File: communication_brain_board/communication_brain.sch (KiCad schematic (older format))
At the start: 27 parts, among them J1 UART, J2 Batt, J3 RS485, J4 CAN, SW1 Reset, SW2 Programm, U1 LM2576HVT-ADJ, U2 L78L33_TO92, U3 ESP-12E, U4 MAX485E, U5 MCP2515-xSO

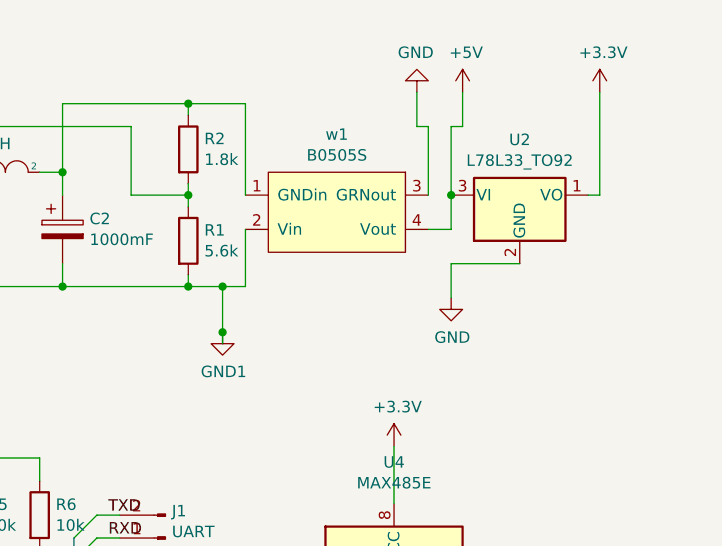
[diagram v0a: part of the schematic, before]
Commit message: fixed scheme
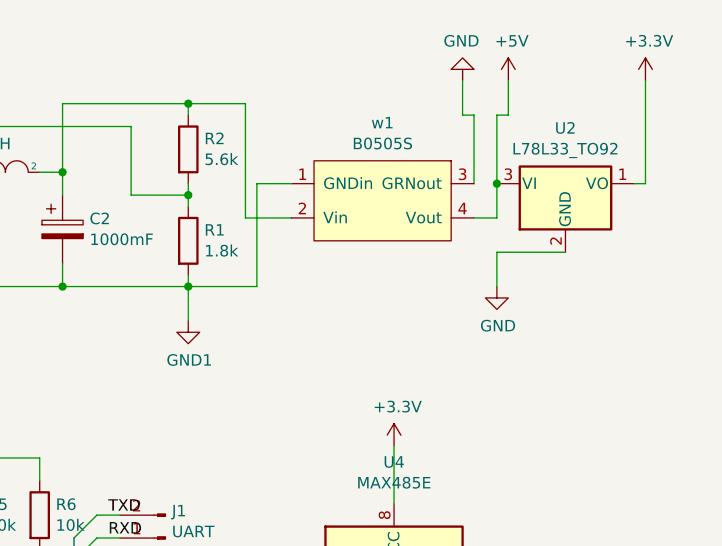
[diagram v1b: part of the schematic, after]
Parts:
- R1: value 5.6k -> 1.8k
- R2: value 1.8k -> 5.6k
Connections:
- net -BATT: now also w1.1 (GNDin); no longer w1.2 (Vin)
- net at C2.1, L1.2, R2.1: now also w1.2 (Vin); no longer w1.1 (GNDin)
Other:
- moved on the sheet: U2, w1
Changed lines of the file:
@@
 P 5500 2100
 F 0 "R1" H 5570 2146 50  0000 L CNN
-F 1 "5.6k" H 5570 2055 50  0000 L CNN
+F 1 "1.8k" H 5570 2055 50  0000 L CNN
 F 2 "Resistor_THT:R_Axial_DIN0207_L6.3mm_D2.5mm_P10.16mm_Horizontal" V 5430 2100 50  0001 C CNN
 F 3 "~" H 5500 2100 50  0001 C CNN
@@
 P 5500 1700
 F 0 "R2" H 5570 1746 50  0000 L CNN
-F 1 "1.8k" H 5570 1655 50  0000 L CNN
+F 1 "5.6k" H 5570 1655 50  0000 L CNN
 F 2 "Resistor_THT:R_Axial_DIN0207_L6.3mm_D2.5mm_P10.16mm_Horizontal" V 5430 1700 50  0001 C CNN
 F 3 "~" H 5500 1700 50  0001 C CNN
@@
 L power:GND1 #PWR0112
 U 1 1 6074119C
-P 5650 2500
-F 0 "#PWR0112" H 5650 2250 50  0001 C CNN
-F 1 "GND1" H 5655 2327 50  0000 C CNN
-F 2 "" H 5650 2500 50  0001 C CNN
-F 3 "" H 5650 2500 50  0001 C CNN
-	1    5650 2500
-	1    0    0    -1
-$EndComp
-Wire Wire Line
-	7300 1900 7300 1450
-Wire Wire Line
-	7250 1900 7300 1900
+P 5500 2450
+F 0 "#PWR0112" H 5500 2200 50  0001 C CNN
+F 1 "GND1" H 5505 2277 50  0000 C CNN
+F 2 "" H 5500 2450 50  0001 C CNN
+F 3 "" H 5500 2450 50  0001 C CNN
+	1    5500 2450
+	1    0    0    -1
+$EndComp
+Wire Wire Line
+	7500 1850 7500 1400
+Wire Wire Line
+	7450 1850 7500 1850
 $Comp
 L power:+3.3V #PWR0105
 U 1 1 600626C6
-P 7300 1450
-F 0 "#PWR0105" H 7300 1300 50  0001 C CNN
-F 1 "+3.3V" H 7315 1623 50  0000 C CNN
-F 2 "" H 7300 1450 50  0001 C CNN
-F 3 "" H 7300 1450 50  0001 C CNN
-	1    7300 1450
+P 7500 1400
+F 0 "#PWR0105" H 7500 1250 50  0001 C CNN
+F 1 "+3.3V" H 7515 1573 50  0000 C CNN
+F 2 "" H 7500 1400 50  0001 C CNN
+F 3 "" H 7500 1400 50  0001 C CNN
+	1    7500 1400
 	1    0    0    -1
 $EndComp
@@
 L Regulator_Linear:L78L33_TO92 U2
 U 1 1 6005D69D
-P 6950 1900
-F 0 "U2" H 6950 2142 50  0000 C CNN
-F 1 "L78L33_TO92" H 6950 2051 50  0000 C CNN
-F 2 "Package_TO_SOT_THT:TO-92_Inline" H 6950 2125 50  0001 C CIN
-F 3 "http://www.st.com/content/ccc/resource/technical/document/datasheet/15/55/e5/aa/23/5b/43/fd/CD00000446.pdf/files/CD00000446.pdf/jcr:content/translations/en.CD00000446.pdf" H 6950 1850 50  0001 C CNN
-	1    6950 1900
+P 7150 1850
+F 0 "U2" H 7150 2092 50  0000 C CNN
+F 1 "L78L33_TO92" H 7150 2001 50  0000 C CNN
+F 2 "Package_TO_SOT_THT:TO-92_Inline" H 7150 2075 50  0001 C CIN
+F 3 "http://www.st.com/content/ccc/resource/technical/document/datasheet/15/55/e5/aa/23/5b/43/fd/CD00000446.pdf/files/CD00000446.pdf/jcr:content/translations/en.CD00000446.pdf" H 7150 1800 50  0001 C CNN
+	1    7150 1850
 	1    0    0    -1
 $EndComp
@@
 L power:+5V #PWR0104
 U 1 1 6005BBEE
-P 6700 1450
-F 0 "#PWR0104" H 6700 1300 50  0001 C CNN
-F 1 "+5V" H 6715 1623 50  0000 C CNN
-F 2 "" H 6700 1450 50  0001 C CNN
-F 3 "" H 6700 1450 50  0001 C CNN
-	1    6700 1450
+P 6900 1400
+F 0 "#PWR0104" H 6900 1250 50  0001 C CNN
+F 1 "+5V" H 6915 1573 50  0000 C CNN
+F 2 "" H 6900 1400 50  0001 C CNN
+F 3 "" H 6900 1400 50  0001 C CNN
+	1    6900 1400
 	1    0    0    -1
 $EndComp
@@
 L power:GND #PWR0103
 U 1 1 60032A9B
-P 6650 2350
-F 0 "#PWR0103" H 6650 2100 50  0001 C CNN
-F 1 "GND" H 6655 2177 50  0000 C CNN
-F 2 "" H 6650 2350 50  0001 C CNN
-F 3 "" H 6650 2350 50  0001 C CNN
-	1    6650 2350
+P 6850 2300
+F 0 "#PWR0103" H 6850 2050 50  0001 C CNN
+F 1 "GND" H 6855 2127 50  0000 C CNN
+F 2 "" H 6850 2300 50  0001 C CNN
+F 3 "" H 6850 2300 50  0001 C CNN
+	1    6850 2300
 	1    0    0    -1
 $EndComp
@@
 L Converter_DCDC:B0505S w1
 U 1 1 606C6681
-P 6150 1750
-F 0 "w1" H 6150 1865 50  0000 C CNN
-F 1 "B0505S" H 6150 1774 50  0000 C CNN
-F 2 "" H 6150 1750 50  0001 C CNN
-F 3 "" H 6150 1750 50  0001 C CNN
-	1    6150 1750
-	1    0    0    -1
-$EndComp
-Wire Wire Line
-	6550 2050 6650 2050
-Wire Wire Line
-	6650 2050 6650 1900
-Wire Wire Line
-	6950 2200 6650 2200
-Wire Wire Line
-	6650 2200 6650 2350
+P 6350 1700
+F 0 "w1" H 6350 1815 50  0000 C CNN
+F 1 "B0505S" H 6350 1724 50  0000 C CNN
+F 2 "" H 6350 1700 50  0001 C CNN
+F 3 "" H 6350 1700 50  0001 C CNN
+	1    6350 1700
+	1    0    0    -1
+$EndComp
+Wire Wire Line
+	6750 2000 6850 2000
+Wire Wire Line
+	6850 2000 6850 1850
+Wire Wire Line
+	7150 2150 6850 2150
+Wire Wire Line
+	6850 2150 6850 2300
 $Comp
 L power:GND #PWR0113
 U 1 1 607A766E
-P 6500 1450
-F 0 "#PWR0113" H 6500 1200 50  0001 C CNN
-F 1 "GND" H 6505 1277 50  0000 C CNN
-F 2 "" H 6500 1450 50  0001 C CNN
-F 3 "" H 6500 1450 50  0001 C CNN
-	1    6500 1450
+P 6700 1400
+F 0 "#PWR0113" H 6700 1150 50  0001 C CNN
+F 1 "GND" H 6705 1227 50  0000 C CNN
+F 2 "" H 6700 1400 50  0001 C CNN
+F 3 "" H 6700 1400 50  0001 C CNN
+	1    6700 1400
 	-1   0    0    1
 $EndComp
 Wire Wire Line
-	6550 1900 6550 1600
-Wire Wire Line
-	6550 1600 6500 1600
-Wire Wire Line
-	6500 1600 6500 1450
-Wire Wire Line
-	6650 1900 6650 1600
-Wire Wire Line
-	6650 1600 6700 1600
-Wire Wire Line
-	6700 1600 6700 1450
-Connection ~ 6650 1900
-Wire Wire Line
-	5750 2050 5750 2300
-Wire Wire Line
-	5650 2300 5500 2300
+	6750 1850 6750 1550
+Wire Wire Line
+	6750 1550 6700 1550
+Wire Wire Line
+	6700 1550 6700 1400
+Wire Wire Line
+	6850 1850 6850 1550
+Wire Wire Line
+	6850 1550 6900 1550
+Wire Wire Line
+	6900 1550 6900 1400
+Connection ~ 6850 1850
 Connection ~ 5500 2300
-Wire Wire Line
-	5650 2550 5650 2500
-Connection ~ 5650 2500
-Wire Wire Line
-	5650 2500 5650 2300
-Wire Wire Line
-	5750 1900 5750 1500
 Connection ~ 5500 1500
 Wire Wire Line
-	5750 2300 5650 2300
-Connection ~ 5650 2300
-Wire Wire Line
 	5500 1500 5750 1500
+Wire Wire Line
+	5950 2000 5750 2000
+Wire Wire Line
+	5750 2000 5750 1500
+Wire Wire Line
+	5950 1850 5800 1850
+Wire Wire Line
+	5800 1850 5800 2300
+Wire Wire Line
+	5500 2300 5800 2300
+Wire Wire Line
+	5500 2450 5500 2300
 Wire Bus Line
 	4700 3550 4700 4200

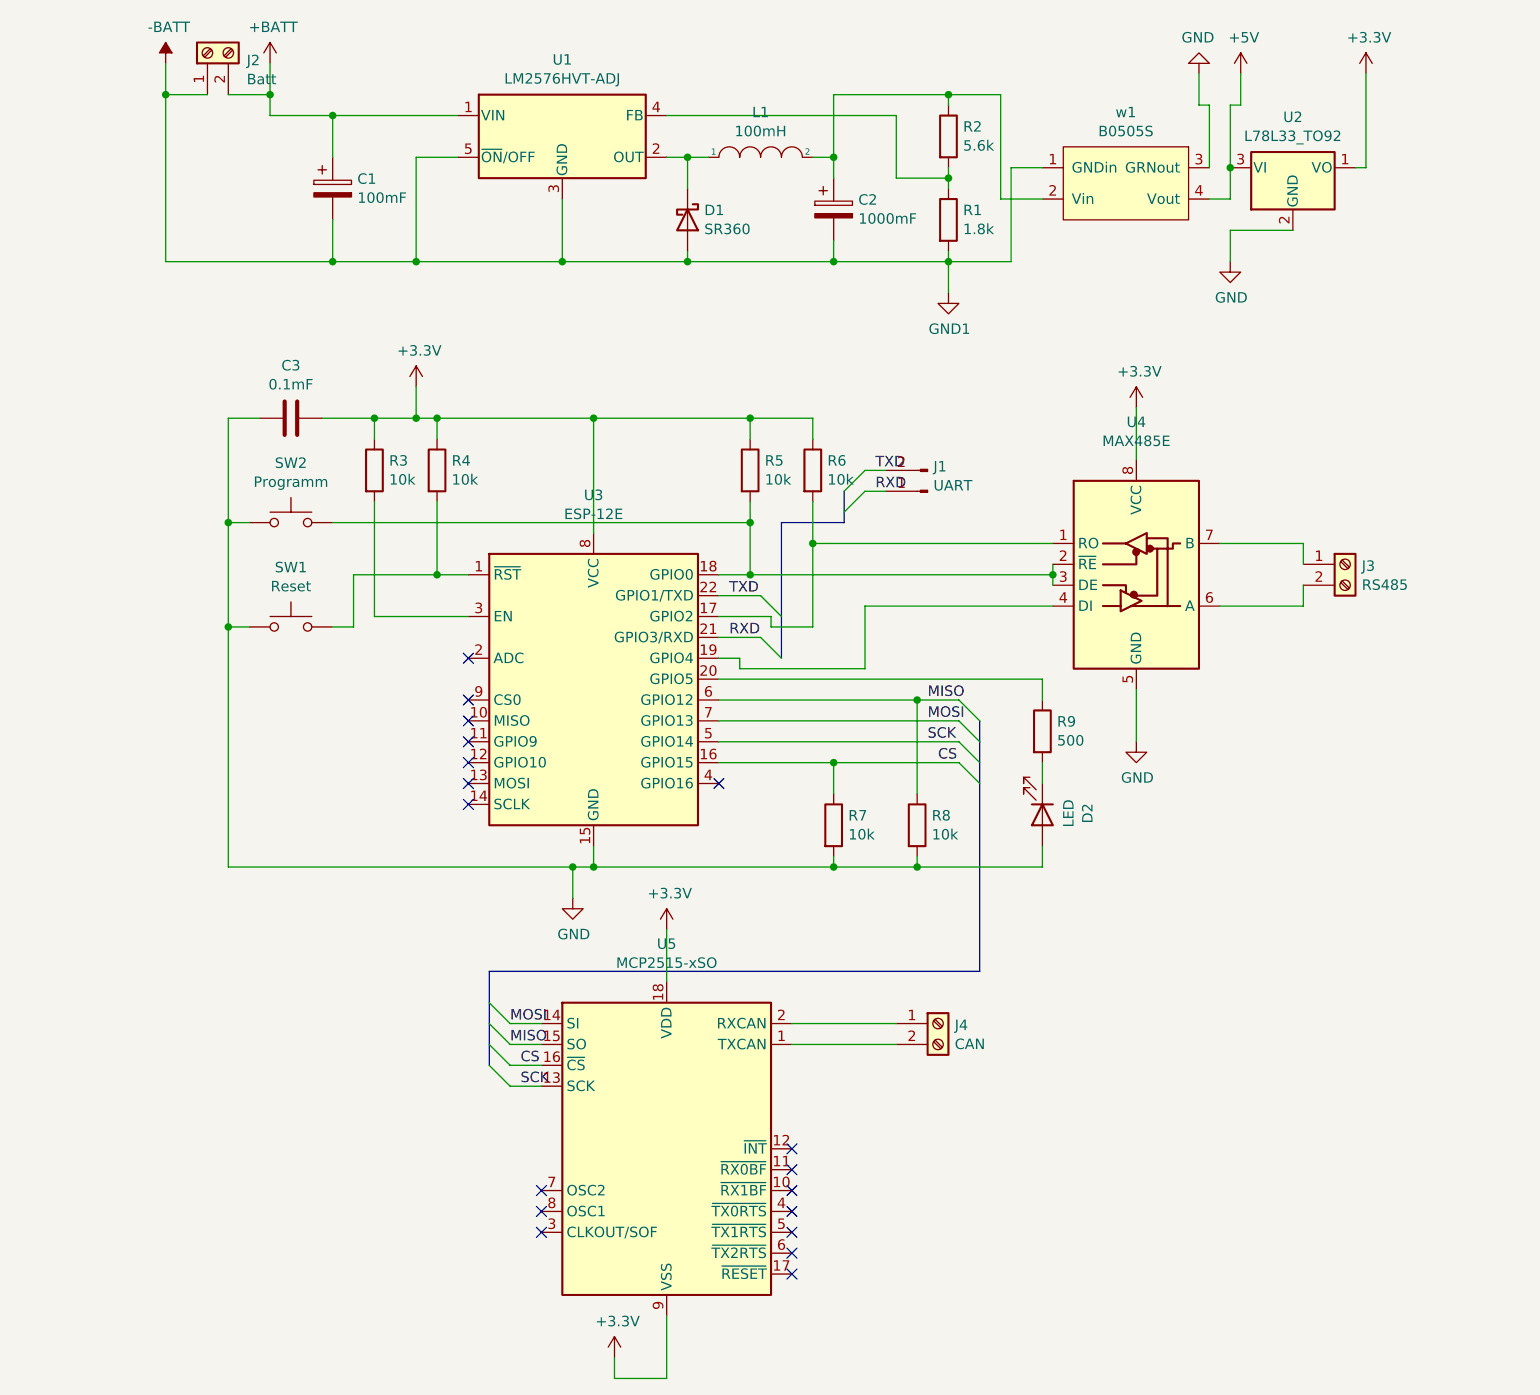
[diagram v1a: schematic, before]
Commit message: Schema update, little adjustments
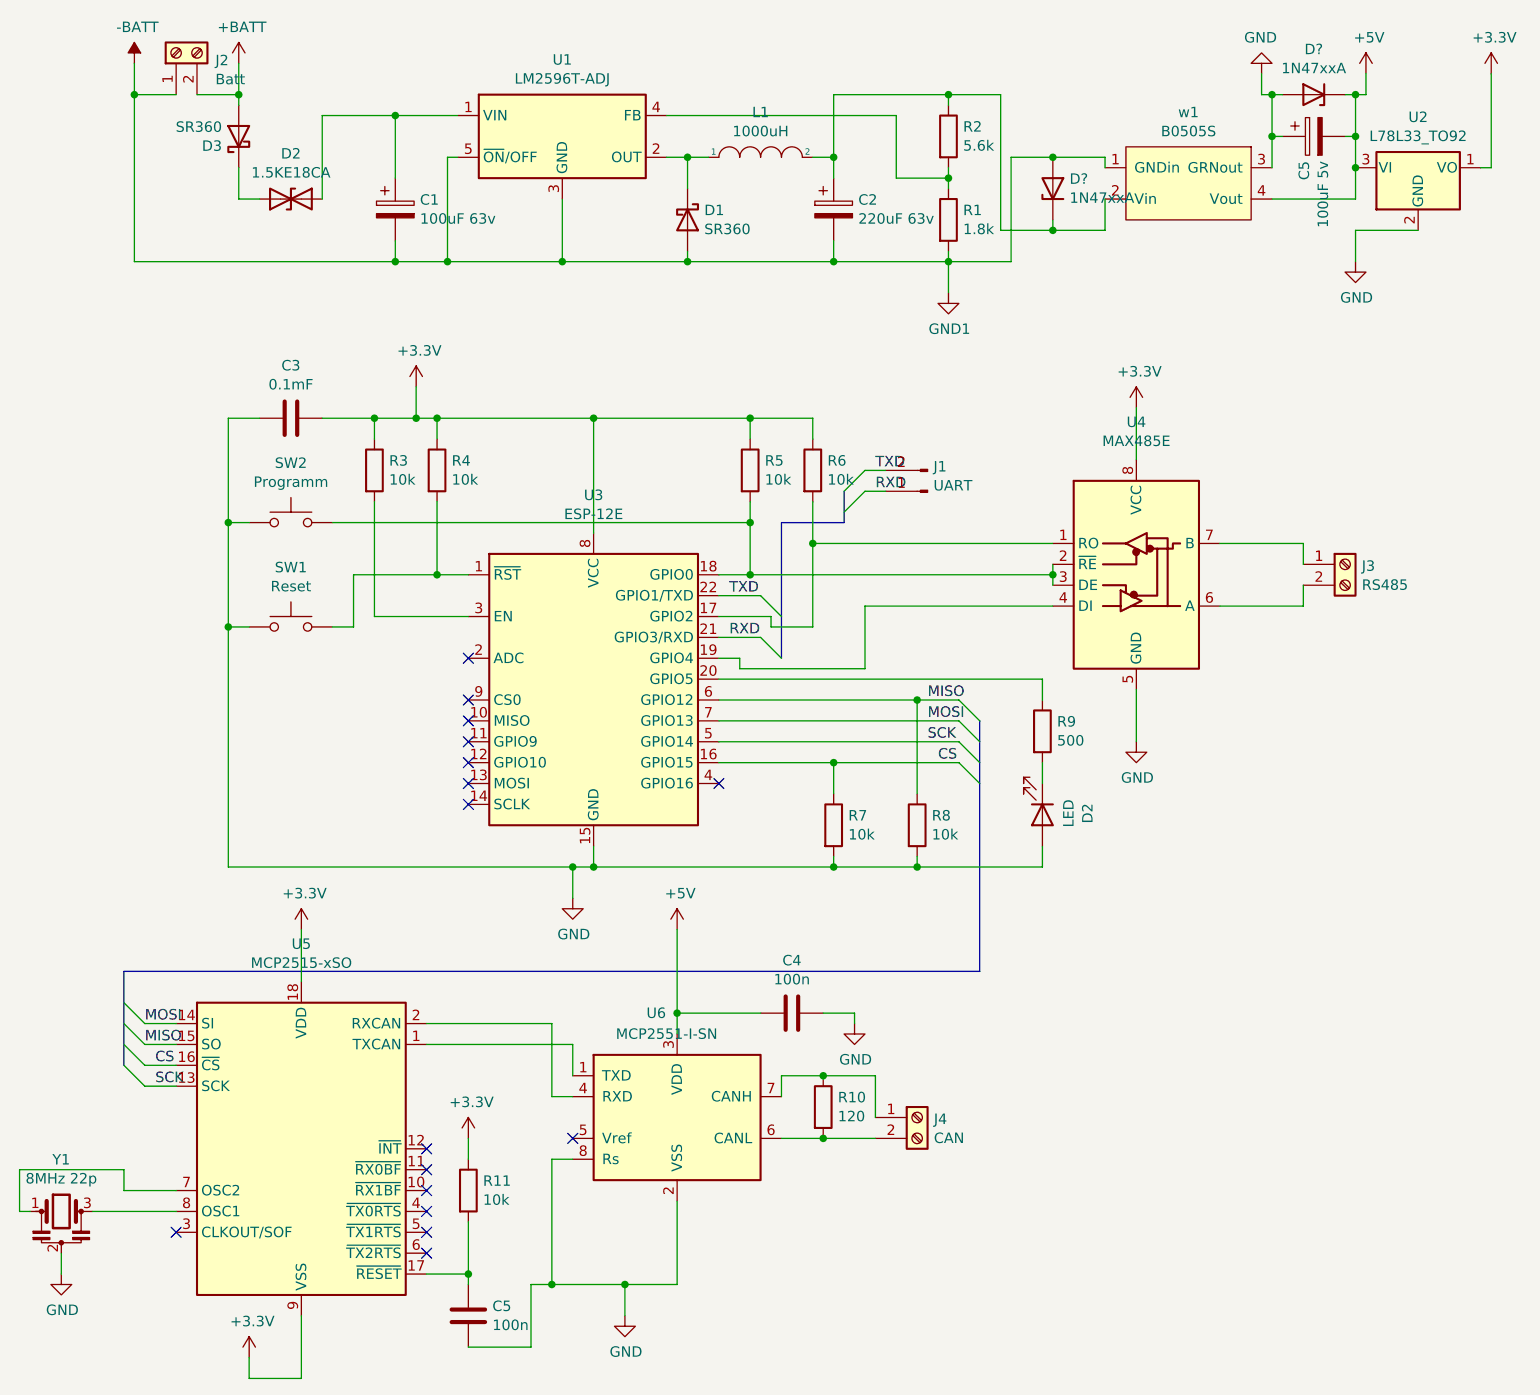
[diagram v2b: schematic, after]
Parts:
- removed U1: LM2576HVT-ADJ, Package_TO_SOT_THT:TO-220-5_Vertical, symbol Regulator_Switching:LM2576HVT-ADJ
- added C4, C5: 100n, symbol Device:C
- added C5: 100uF 5v, Capacitor_THT:C_Radial_D5.0mm_H5.0mm_P2.00mm, symbol Device:CP
- added D2: 1.5KE18CA, Diode_THT:D_DO-201AE_P15.24mm_Horizontal, symbol Diode:1.5KExxCA
- added D3: SR360, Diode_THT:D_DO-201AD_P15.24mm_Horizontal, symbol Diode:1N5822
- added D? (x2): 1N47xxA, Diode_THT:D_DO-41_SOD81_P10.16mm_Horizontal, symbol Diode:1N47xxA
- added R10: 120, Resistor_SMD:R_2010_5025Metric, symbol Device:R
- added R11: 10k, Resistor_SMD:R_2010_5025Metric, symbol Device:R
- added U1: LM2596T-ADJ, Package_TO_SOT_THT:TO-220-5_P3.4x3.7mm_StaggerOdd_Lead3.8mm_Vertical, symbol Regulator_Switching:LM2596T-ADJ
- added U6: MCP2551-I-SN, Package_SO:SOIC-8_3.9x4.9mm_P1.27mm, symbol Interface_CAN_LIN:MCP2551-I-SN
- added Y1: 8MHz 22p, symbol Device:Resonator
- C1: value 100mF -> 100uF 63v
- C2: value 1000mF -> 220uF 63v
- L1: value 100mH -> 1000uH
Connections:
- net +3V3: now also R11.1
- net +5V: now also C4.2, C5.2, D?.1 (K), U6.3 (VDD)
- net +BATT: now also D3.2 (A); no longer C1.1
- net -BATT: now also D?.2 (A), U1.3 (GND), U1.5 (~ON~/OFF)
- net GND: now also C4.1, C5.1, C5.1, D?.2 (A), U6.2 (VSS), U6.8 (Rs), Y1.2
- net at D1.1 (K), L1.1: now also U1.2 (OUT)
- net at R1.1, R2.2: now also U1.4 (FB)
- net at C2.1, L1.2, R2.1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: now also D?.1 (K)
- net at J4.1 (Pin_1): now also R10.1, U6.7 (CANH); no longer U5.2 (RXCAN)
- net at J4.2 (Pin_2): now also R10.2, U6.6 (CANL); no longer U5.1 (TXCAN)
- net at U5.17 (~RESET): now also C5.2, R11.2
- net at U5.7 (OSC2): now also Y1.1
- net at U5.8 (OSC1): now also Y1.3
- new net: C1.1, D2.2 (A2), U1.1 (VIN)
- new net: U5.1 (TXCAN), U6.1 (TXD)
- new net: U5.2 (RXCAN), U6.4 (RXD)
- new net: D2.1 (A1), D3.1 (K)
- no-connect marks 18 -> 16
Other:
- moved on the sheet: C1, J2, J4, U2, U5, w1
